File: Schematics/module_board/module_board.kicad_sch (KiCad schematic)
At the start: 31 parts, among them J1 Conn_01x01_Male, J10 Conn_01x02_Male, J2 Conn_01x01_Male, J3 Conn_01x01_Male, J4 Conn_01x01_Male, J5 Conn_01x06_Male, J6 Conn_01x02_Male, J7 Conn_01x02_Male, J8 Conn_01x04_Male, J9 Conn_01x02_Male, U1 RP2040, U2 W25Q16JVSSIQ, Y1 ABLS-12.000MHZ-B4-T

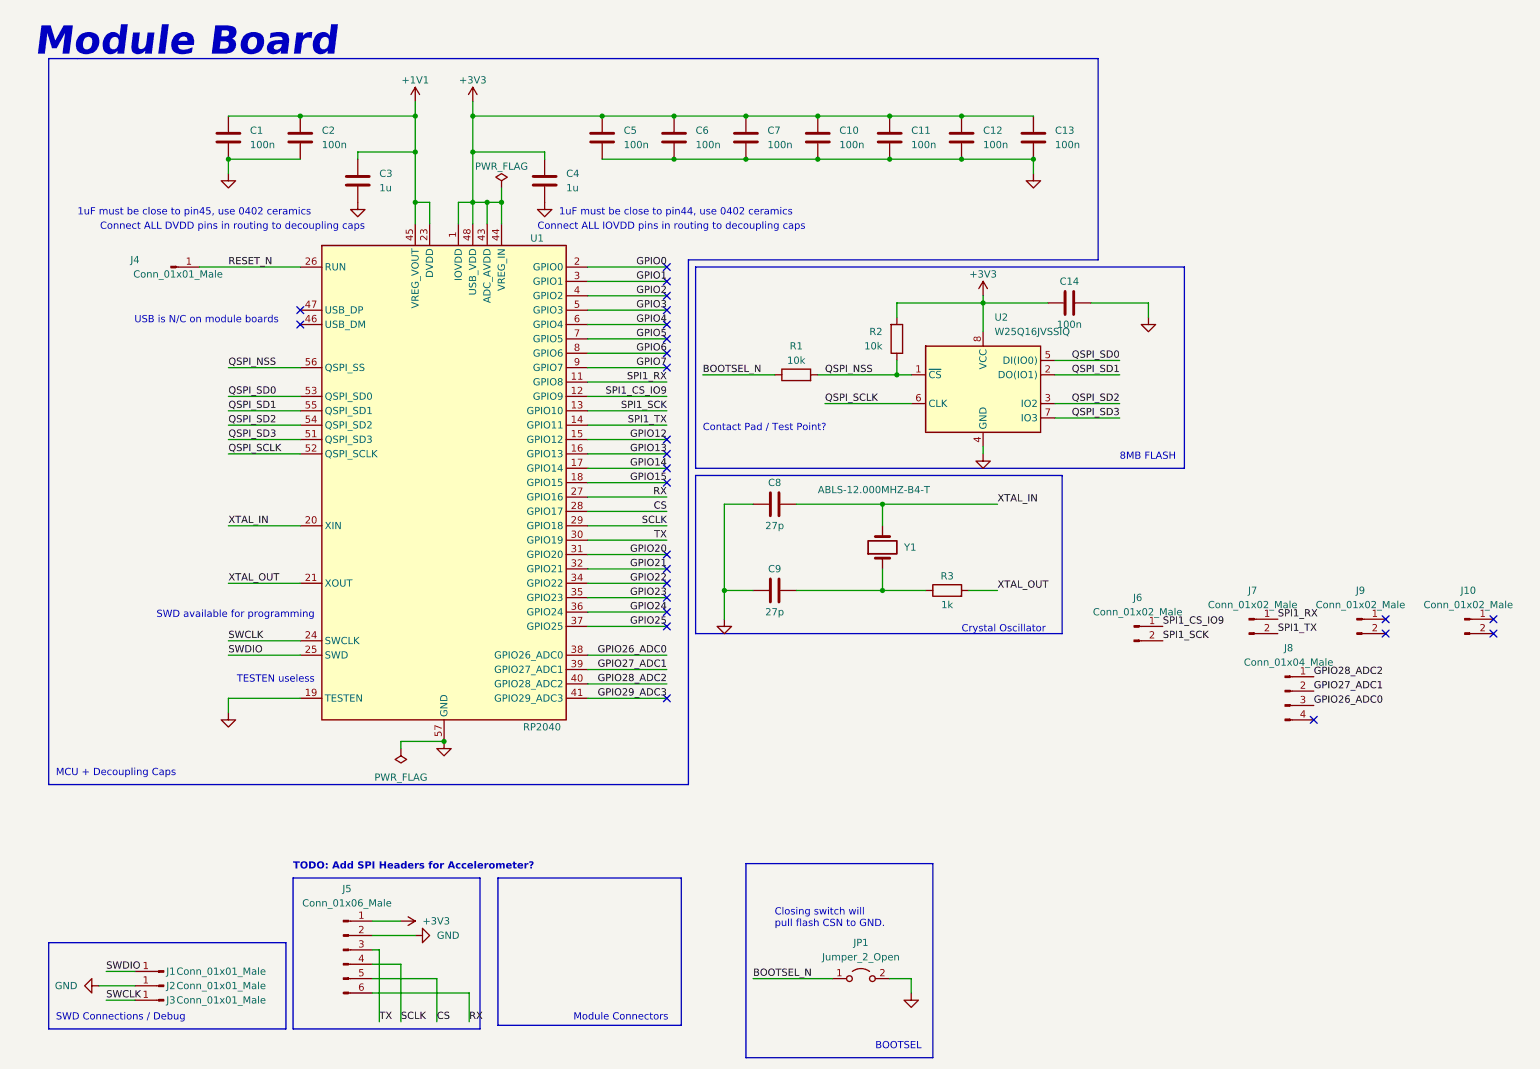
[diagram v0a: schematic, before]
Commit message: Mod board finalizations
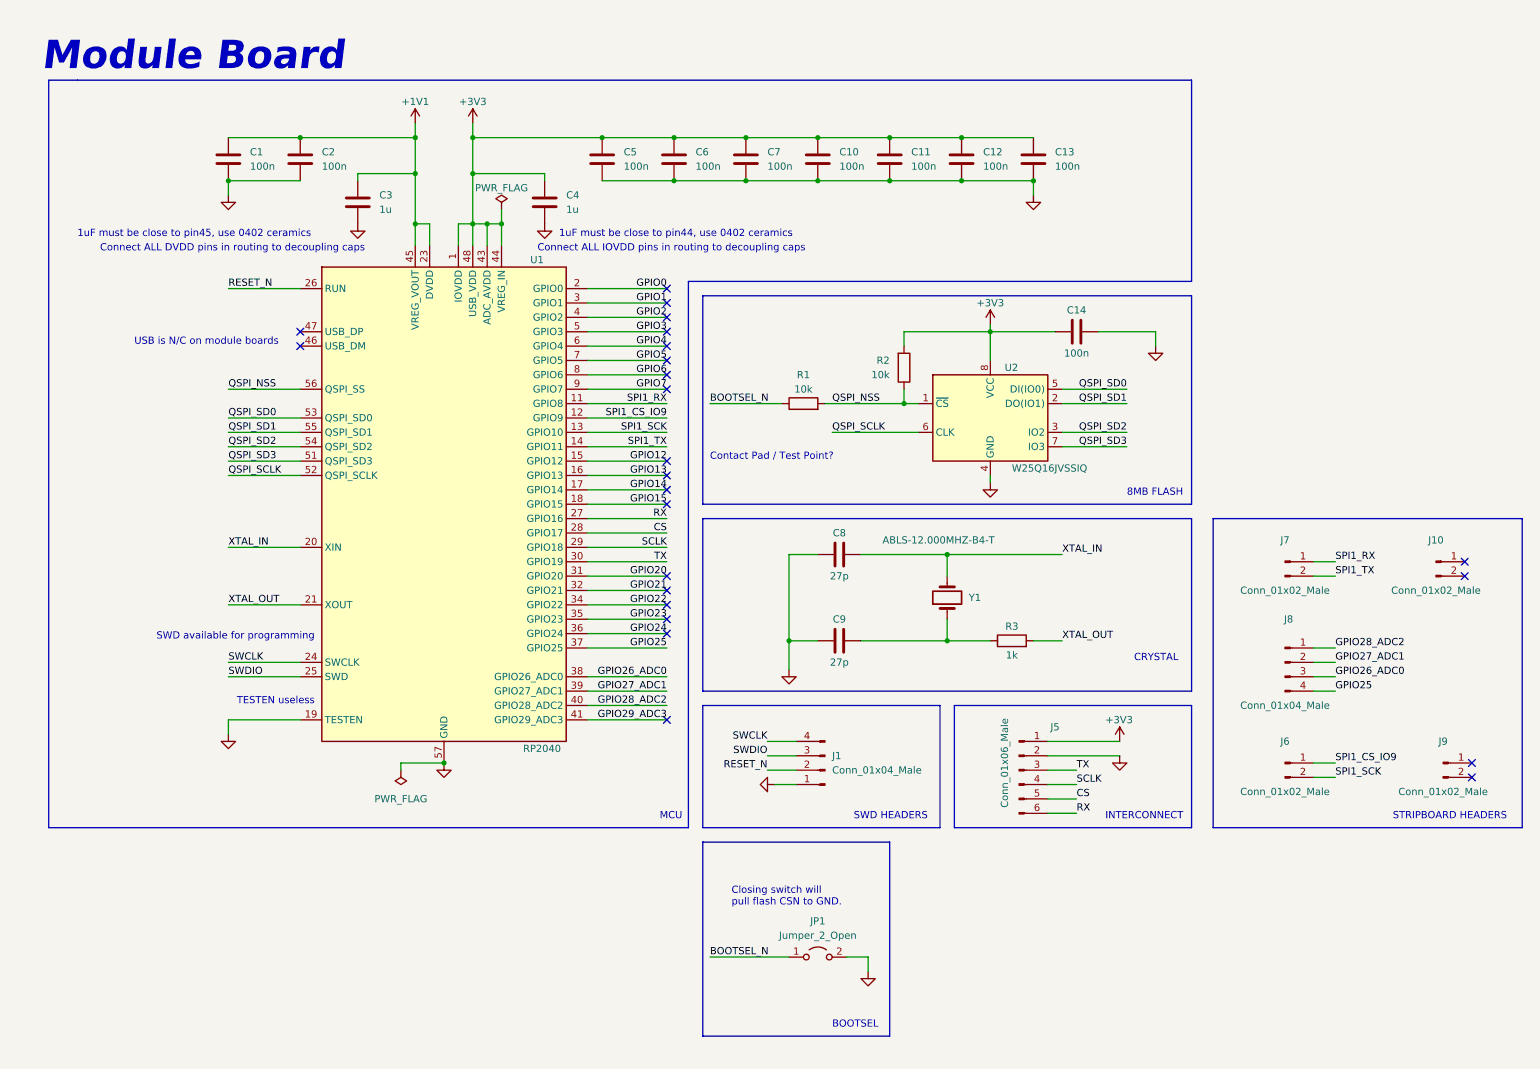
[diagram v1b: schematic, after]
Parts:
- removed J1, J2, J3, J4: Conn_01x01_Male, TestPoint:TestPoint_Pad_D1.0mm, symbol Connector:Conn_01x01_Male
- added J1: Conn_01x04_Male, Connector_PinHeader_2.54mm:PinHeader_1x04_P2.54mm_Vertical, symbol Connector:Conn_01x04_Male
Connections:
- net GND: now also J1.1 (Pin_1)
- net GPIO25: now also J8.4 (Pin_4)
- net RESET_N: now also J1.2 (Pin_2)
- net SWCLK: now also J1.4 (Pin_4)
- net SWDIO: now also J1.3 (Pin_3)
- no-connect marks 26 -> 24
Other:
- note added: "CRYSTAL"
- note added: "INTERCONNECT"
- note added: "MCU"
- note added: "STRIPBOARD HEADERS"
- note added: "SWD HEADERS"
- note removed: "Crystal Oscillator"
- note removed: "MCU + Decoupling Caps"
- note removed: "Module Connectors"
- note removed: "SWD Connections / Debug"
- note removed: "TODO: Add SPI Headers for Accelerometer?"
- moved on the sheet: C1, C10, C11, C12, C13, C14, C2, C3, C4, C5, C6, C7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
